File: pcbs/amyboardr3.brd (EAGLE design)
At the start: 100 x 80 mm, 109 parts, among them M13 M2.5, M14 M2.5, M15 M2.5, M16 M2.5, Q2 S8050, Q5 S8050, SW2 JS102011JAQN, U1 PCM9211PT, U13 HX3608, U14 CH340K, U15 H11L1SR2M, U16 SPX3819, U2 ESP32­S2­SOLO, Y1 ABM10W-22.5792MHZ-8-K1Z-T3

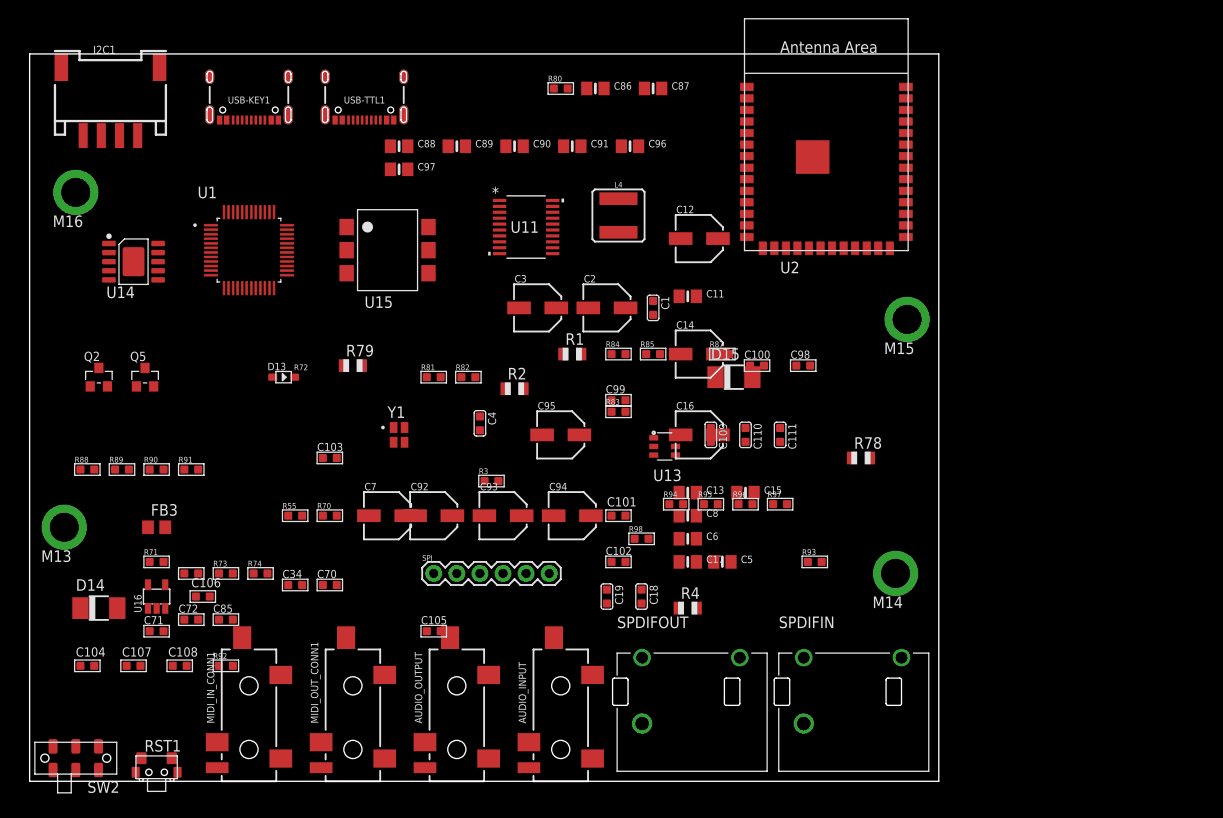
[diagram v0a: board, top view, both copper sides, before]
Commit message: moving to 3.5mm jacks for everything
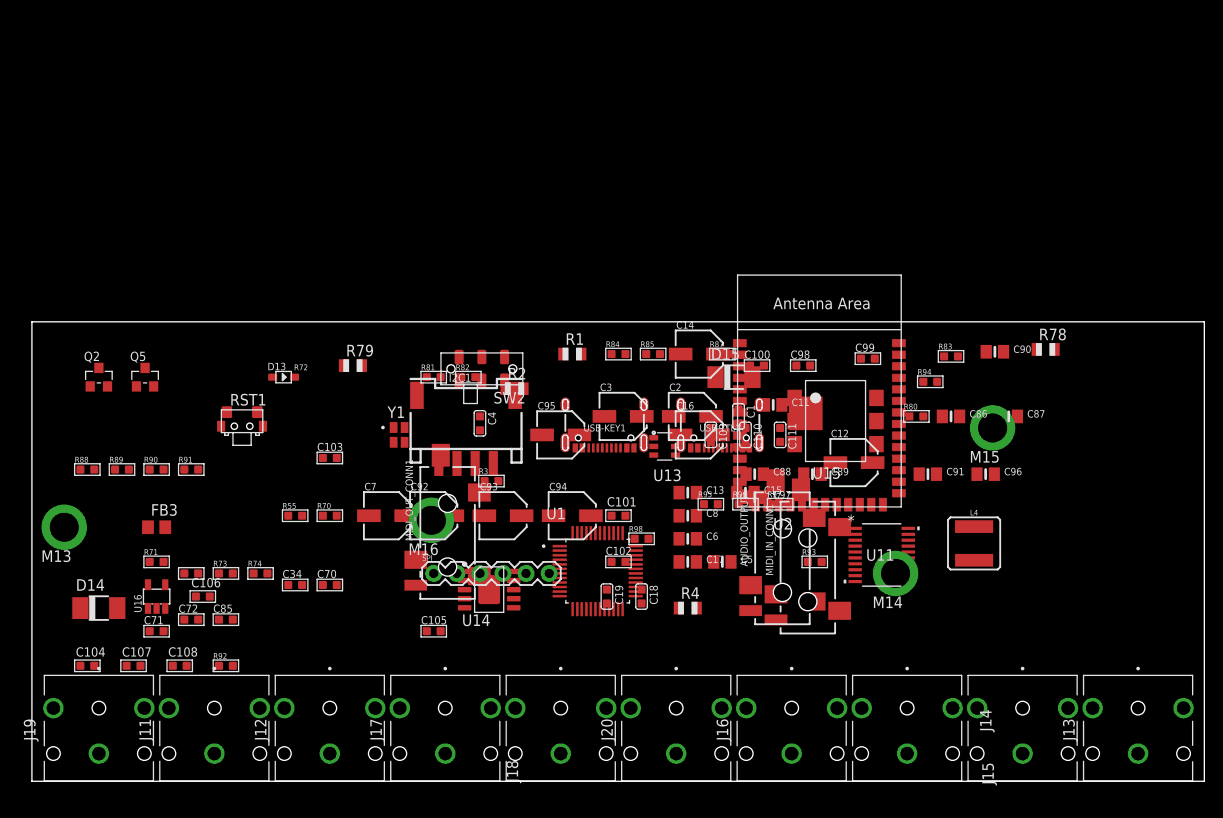
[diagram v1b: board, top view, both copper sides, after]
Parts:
- removed AUDIO_INPUT: 19269, microbuilder:4UCONN_19269
- removed SPDIFIN, SPDIFOUT: PJRAS1X1S01, PJRAS1X1S01:SWITCHCRAFT_PJRAS1X1S01
- added J11, J12, J13, J14, J15, J16, J17, J18, J19, J20: SJ1-3543, SJ1-3543:CUI_SJ1-3543
- moved MIDI_IN_CONN1 63.6 mm to (85.6, 16.3)
- moved SW2 61.9 mm to (49.7, 45.4)
- moved C90 57.5 mm to (106.2, 47.2)
- moved C86 53.2 mm to (101.3, 40.1)
- moved C87 53.2 mm to (107.7, 40.1)
- moved C88 53.2 mm to (79.8, 33.8)
- moved C91 53.2 mm to (98.8, 33.8)
- moved C96 53.2 mm to (105.2, 33.8)
- moved C97 53.2 mm to (79.8, 31.2)
- moved I2C1 53.2 mm to (48.0, 35.1)
- moved L4 53.2 mm to (103.9, 26.2)
- moved M16 53.2 mm to (44.2, 28.7)
- moved PCM5101 53.2 mm to (93.7, 24.9)
- moved R80 53.2 mm to (97.5, 40.1)
- moved U14 53.2 mm to (50.5, 21.1)
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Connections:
- net AGND: now also J11.1; no longer AUDIO_INPUT.1
- net BCLK: now also J20.2
- net GND: no longer SPDIFIN.G, SPDIFIN.S, SPDIFOUT.G, SPDIFOUT.S
- net LIN: now also J11.2; no longer AUDIO_INPUT.2, AUDIO_INPUT.4
- net LINX: now also J20.1
- net RIN: now also J11.3; no longer AUDIO_INPUT.3, AUDIO_INPUT.5
- net RINX: now also J20.3
- net SPDIFIN_SIGNAL: no longer SPDIFIN.T
- net SPDIFOUT_SIGNAL: no longer SPDIFOUT.T
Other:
- board size 100 x 80 mm -> 129 x 50.5 mm
